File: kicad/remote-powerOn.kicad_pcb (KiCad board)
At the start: 2 copper layers, 43 x 43 mm, 17 parts, among them K1 LMR2-3D, Q1 BC517

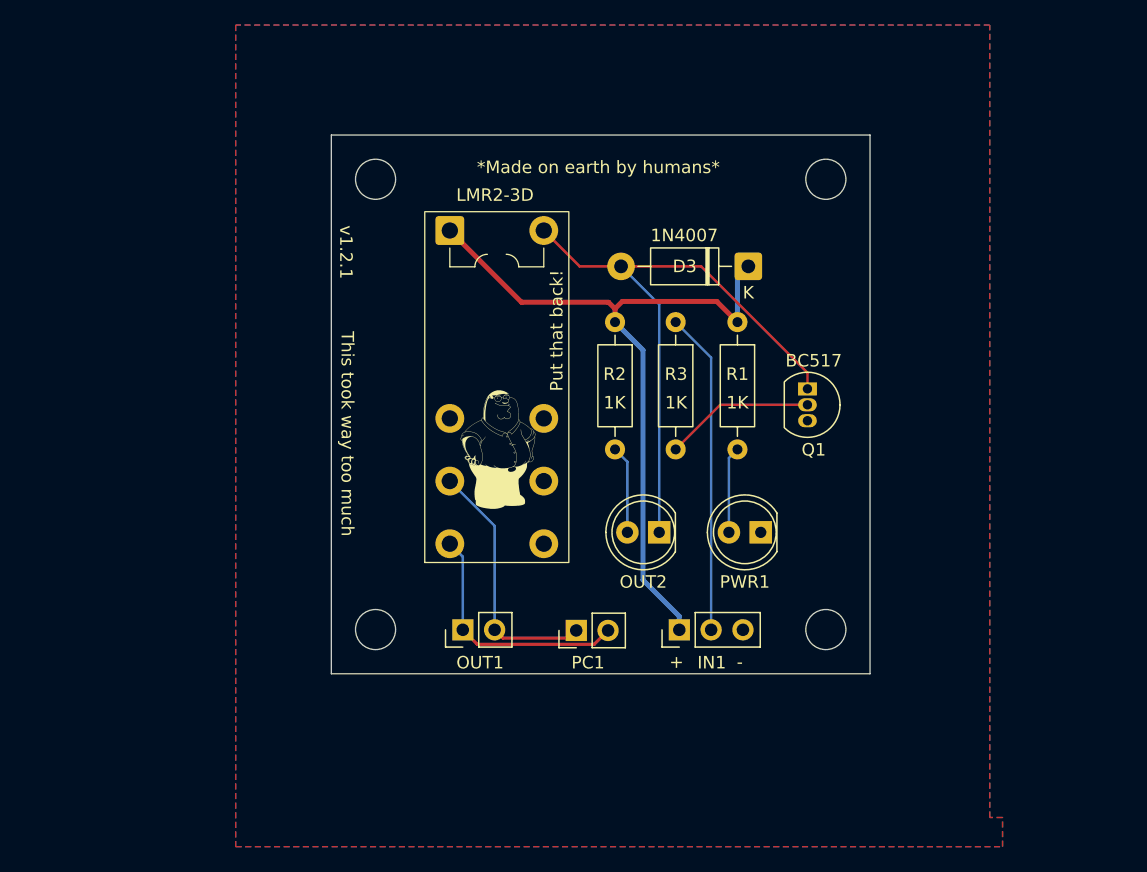
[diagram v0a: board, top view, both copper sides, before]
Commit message: v1.3.0
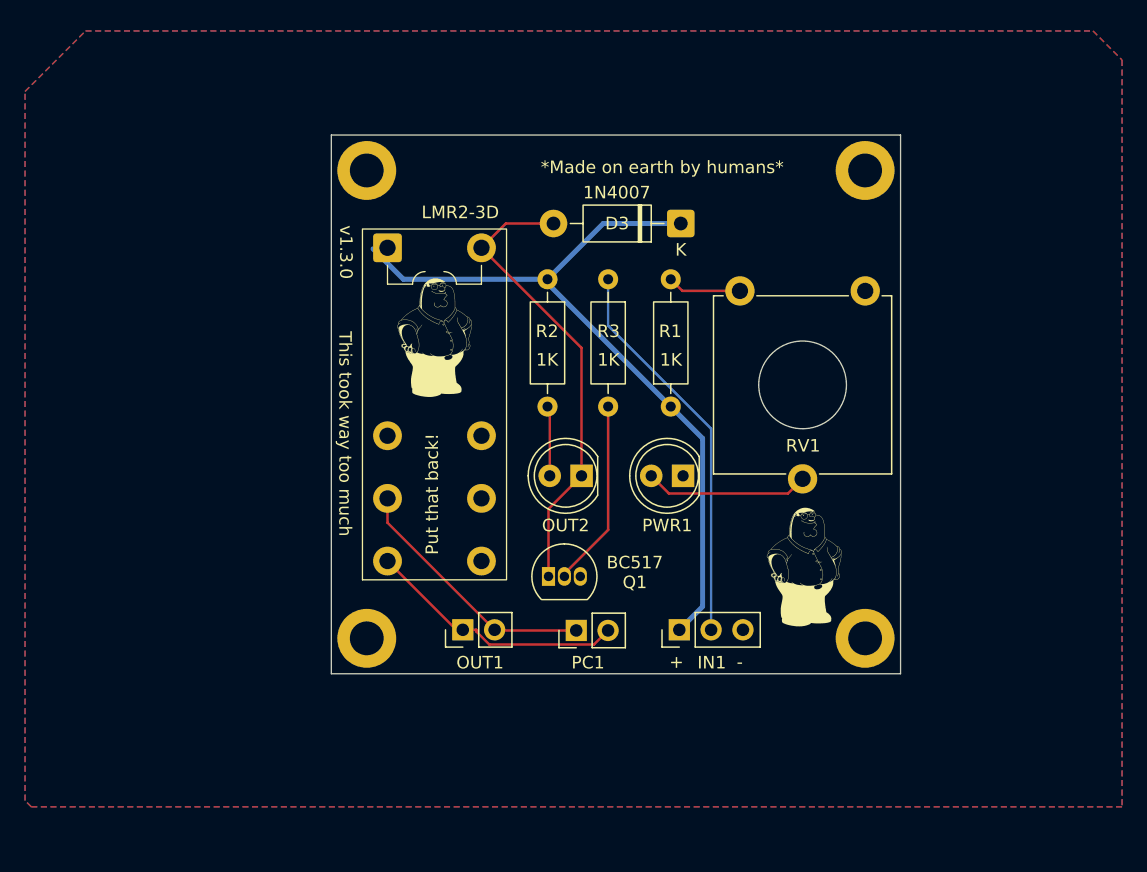
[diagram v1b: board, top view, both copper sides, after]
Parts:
- removed HOLE1, HOLE2, HOLE3, REF**: MountingHole_3.2mm_M3, MountingHole:MountingHole_3.2mm_M3
- added G***: LOGO, SilkScreen:Peter_Image, F.Cu at (154.9, 89.3)
- added H1: MountingHole_Pad, MountingHole:MountingHole_2.7mm_M2.5_DIN965_Pad, F.Cu at (159.8, 57.6)
- added H2: MountingHole_Pad, MountingHole:MountingHole_2.7mm_M2.5_DIN965_Pad, F.Cu at (159.8, 95.0)
- added H3: MountingHole_Pad, MountingHole:MountingHole_2.7mm_M2.5_DIN965_Pad, F.Cu at (120.0, 95.0)
- added H4: MountingHole_Pad, MountingHole:MountingHole_2.7mm_M2.5_DIN965_Pad, F.Cu at (120.0, 57.6)
- added RV1: CA14NV12,5-10KA2020, Potentiometer_THT:Potentiometer_ACP_CA14V-15_Vertical_Hole, F.Cu at (149.8, 67.2)
- R1: value 1K -> 1k
- moved Q1 25.5 mm to (134.5, 90.0), turned to 0 degrees
- moved Peter 10.3 mm to (125.4, 71.0)
- moved R1 8.59 mm to (144.3, 76.5), turned to 90 degrees
- moved OUT2 7.67 mm to (137.2, 82.0)
- moved PWR1 7.67 mm to (145.3, 82.0)
- moved R2 6.38 mm to (134.4, 66.3)
- moved R3 6.38 mm to (139.3, 66.3)
- moved D3 6.38 mm to (145.1, 61.9)
- moved K1 5.16 mm to (121.7, 88.8)
- moved refer2 1.75 mm to (140.3, 76.3)
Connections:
- net /GND renamed GND
- R1 pad 2: Net-(PWR1-A) -> Net-(R1-Pad2)
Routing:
- net Net-(D3-A): track 49.5 -> 37.2 mm
- net Net-(PWR1-A): track 6.90 -> 13.1 mm
- net Net-(R1-Pad2): track 0.00 -> 5.91 mm
- net /INPUT: track 25.7 -> 31.4 mm
- net Net-(Q1-B): track 12.0 -> 15.0 mm
- net /VCC: track 59.0 -> 61.2 mm
- net Net-(OUT2-A): track 7.03 -> 5.60 mm
- net /OUT1: track 19.8 -> 20.9 mm
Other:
- board size 43 x 43 mm -> 45.4 x 43 mm
- board text added: "1K"
